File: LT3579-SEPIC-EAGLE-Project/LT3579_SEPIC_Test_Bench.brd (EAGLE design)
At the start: 74 x 58 mm, 160 parts

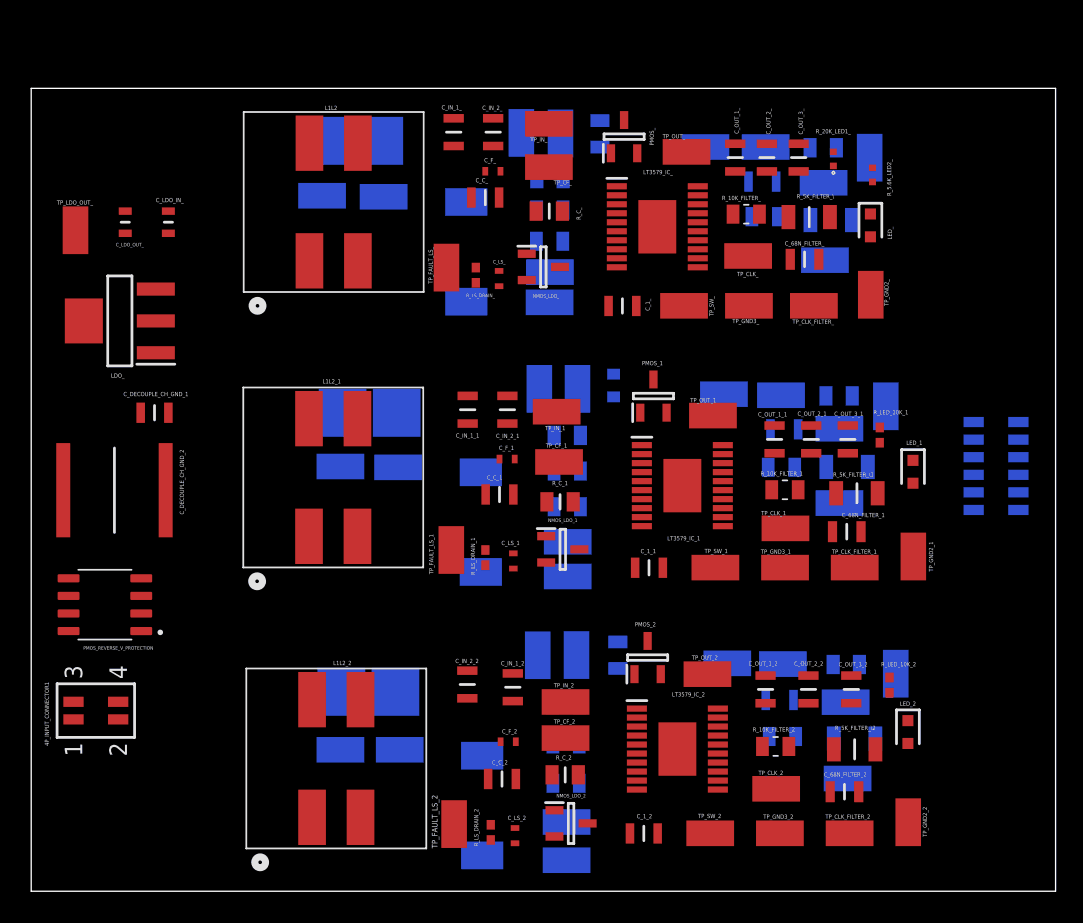
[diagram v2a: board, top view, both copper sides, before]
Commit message: Added new FIles
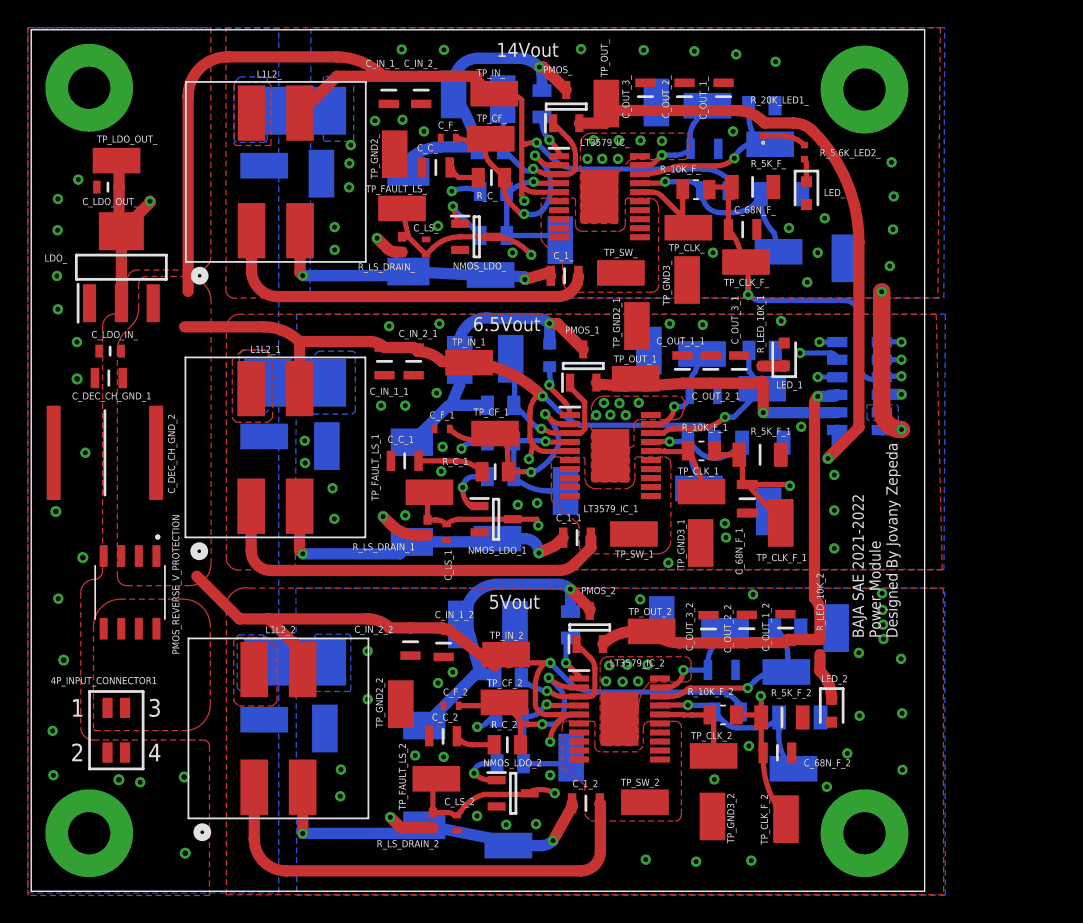
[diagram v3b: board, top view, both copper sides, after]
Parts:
- removed C_68N_FILTER_, C_68N_FILTER_1, C_68N_FILTER_2: CEU4J2X7R1H683K125AE, SamacSys_Parts:CAPC2013X150N
- removed C_DECOUPLE_CH_GND_1: CGA4F4C0G2W222J085AE, SamacSys_Parts:CAPC2012X100N
- removed C_DECOUPLE_CH_GND_2: CGADN3X7R1E476M230LE, SamacSys_Parts:CAPC7563X250N
- removed R_10K_FILTER_, R_10K_FILTER_1, R_10K_FILTER_2: AC0805DR-0710KL, AC0805DR-0710KL:RESC2012X60N
- removed R_5K_FILTER_\, R_5K_FILTER_\1, R_5K_FILTER_\2: RT1206BRD075KL, SamacSys_Parts:RESC3116X65N
- removed TP_CLK_FILTER_, TP_CLK_FILTER_1, TP_CLK_FILTER_2: S1751-46R, S1751-46R:S1751-46R_
- added C_68N_F_, C_68N_F_1, C_68N_F_2: CEU4J2X7R1H683K125AE, SamacSys_Parts:CAPC2013X150N
- added C_DEC_CH_GND_1: CGA4F4C0G2W222J085AE, SamacSys_Parts:CAPC2012X100N
- added C_DEC_CH_GND_2: CGADN3X7R1E476M230LE, SamacSys_Parts:CAPC7563X250N
- added R_10K_F_, R_10K_F_1, R_10K_F_2: AC0805DR-0710KL, AC0805DR-0710KL:RESC2012X60N
- added R_5K_F_, R_5K_F_1, R_5K_F_2: RT1206BRD075KL, SamacSys_Parts:RESC3116X65N
- added TP_CLK_F_, TP_CLK_F_1, TP_CLK_F_2: S1751-46R, S1751-46R:S1751-46R_
- added U$1, U$2, U$3, U$4: THROUGH_HOLE_, THROUGH_HOLE:THROUGH_HOLE
- moved TP_GND2_2 37.6 mm to (26.7, 13.5), turned to 270 degrees
- moved TP_GND2_ 35.9 mm to (26.3, 53.2)
- moved TP_GND2_1 26.0 mm to (43.8, 40.8), turned to 90 degrees
- moved LED_1 12.6 mm to (54.4, 38.8), turned to 90 degrees
- moved C_OUT_3_ 11.9 mm to (44.4, 57.4), turned to 90 degrees
- moved 12P_OUTPUT_CONNECTOR1 11.4 mm to (59.8, 36.5)
- moved TP_GND4_1 11.4 mm to (53.3, 27.4), turned to 90 degrees
- moved C_OUT_3_2 11.2 mm to (48.9, 18.9), turned to 90 degrees
- moved C_LDO_IN_ 10.2 mm to (5.70, 39.0), turned to 180 degrees
- moved TP_SHDN_1 10.2 mm to (48.2, 29.1)
- moved R_LED_10K_1 9.61 mm to (52.8, 37.4), turned to 90 degrees
- moved C_OUT_3_1 9.34 mm to (51.1, 37.7), turned to 90 degrees
- moved C_OUT_2_1 8.84 mm to (49.1, 37.7), turned to 90 degrees
- moved C_OUT_1_1 8.36 mm to (47.0, 37.7), turned to 90 degrees
- moved C_IN_2_1 7.62 mm to (27.6, 38.3)
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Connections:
- removed net 0: C_68N_FILTER_.2, C_68N_FILTER_1.2, C_68N_FILTER_2.2, C_C_.2, C_C_1.2, C_C_2.2, C_F_.2, C_F_1.2, C_F_2.2, C_IN_1_.2, C_IN_1_1.2, C_IN_1_2.2, C_IN_2_.2, C_IN_2_1.2, C_IN_2_2.2, C_LDO_IN_.2, C_LDO_OUT_.2, C_LS_.2, C_LS_1.2, C_LS_2.2, C_OUT_1_.2, C_OUT_1_1.2, C_OUT_1_2.2, C_OUT_2_.2, C_OUT_2_1.2, C_OUT_2_2.2, C_OUT_3_.2, C_OUT_3_1.2, C_OUT_3_2.2, C_SS_.2, C_SS_1.2, C_SS_2.2, L1L2_.4, L1L2_1.4, L1L2_2.4, LED_.2, LED_1.2, LED_2.2, LT3579_IC_.21, LT3579_IC_1.21, LT3579_IC_2.21, NMOS_LDO_.2, NMOS_LDO_1.2, NMOS_LDO_2.2, PMOS_REVERSE_V_PROTECTION.4, R_5K_FILTER_\.2, R_5K_FILTER_\1.2, R_5K_FILTER_\2.2, R_T_.2, R_T_1.2, R_T_2.2, R_UVLO2_.1, R_UVLO2_1.1, R_UVLO2_2.1, TP_GND1_.1, TP_GND1_1.1, TP_GND1_2.1, TP_GND2_.1, TP_GND2_1.1, TP_GND2_2.1, TP_GND3_.1, TP_GND3_1.1, TP_GND3_2.1, TP_GND4_.1, TP_GND4_1.1, TP_GND4_2.1
- removed net GND: 12P_OUTPUT_CONNECTOR1.10, 12P_OUTPUT_CONNECTOR1.12, 12P_OUTPUT_CONNECTOR1.8, LDO_.1, LT3579_IC_.20, LT3579_IC_1.20, LT3579_IC_2.20, R_SHUNT_GND_.2, R_SHUNT_GND_1.2, R_SHUNT_GND_2.2, TP_GND_.1, TP_GND_1.1, TP_GND_2.1
- new net GND_: 12P_OUTPUT_CONNECTOR1.12, C_68N_F_.2, C_C_.2, C_F_.2, C_IN_1_.2, C_IN_2_.2, C_LS_.2, C_OUT_1_.2, C_OUT_2_.2, C_OUT_3_.2, C_SS_.2, L1L2_.4, LED_.2, LT3579_IC_.20, LT3579_IC_.21, NMOS_LDO_.2, R_5K_F_.2, R_SHUNT_GND_.2, R_T_.2, R_UVLO2_.1, TP_GND1_.1, TP_GND2_.1, TP_GND3_.1, TP_GND4_.1, TP_GND_.1
- new net GND_1: 12P_OUTPUT_CONNECTOR1.10, C_68N_F_1.2, C_C_1.2, C_F_1.2, C_IN_1_1.2, C_IN_2_1.2, C_LS_1.2, C_OUT_1_1.2, C_OUT_2_1.2, C_OUT_3_1.2, C_SS_1.2, L1L2_1.4, LED_1.2, LT3579_IC_1.20, LT3579_IC_1.21, NMOS_LDO_1.2, R_5K_F_1.2, R_SHUNT_GND_1.2, R_T_1.2, R_UVLO2_1.1, TP_GND1_1.1, TP_GND2_1.1, TP_GND3_1.1, TP_GND4_1.1, TP_GND_1.1
- new net GND_2: 12P_OUTPUT_CONNECTOR1.8, C_68N_F_2.2, C_C_2.2, C_F_2.2, C_IN_1_2.2, C_IN_2_2.2, C_LS_2.2, C_OUT_1_2.2, C_OUT_2_2.2, C_OUT_3_2.2, C_SS_2.2, L1L2_2.4, LED_2.2, LT3579_IC_2.20, LT3579_IC_2.21, NMOS_LDO_2.2, R_5K_F_2.2, R_SHUNT_GND_2.2, R_T_2.2, R_UVLO2_2.1, TP_GND1_2.1, TP_GND2_2.1, TP_GND3_2.1, TP_GND4_2.1, TP_GND_2.1
- net CH_GND: now also C_DEC_CH_GND_1.1, C_DEC_CH_GND_2.1, C_LDO_IN_.2, C_LDO_OUT_.2, LDO_.1, PMOS_REVERSE_V_PROTECTION.4; no longer C_DECOUPLE_CH_GND_1.1, C_DECOUPLE_CH_GND_2.1
- net CLK_: now also R_10K_F_.1; no longer R_10K_FILTER_.1
- net CLK_1: now also R_10K_F_1.1; no longer R_10K_FILTER_1.1
- net CLK_2: now also R_10K_F_2.1; no longer R_10K_FILTER_2.1
- net CLK_FILTER_OUT_: now also C_68N_F_.1, R_10K_F_.2, R_5K_F_.1, TP_CLK_F_.1; no longer C_68N_FILTER_.1, R_10K_FILTER_.2, R_5K_FILTER_\.1, TP_CLK_FILTER_.1
- net CLK_FILTER_OUT_1: now also C_68N_F_1.1, R_10K_F_1.2, R_5K_F_1.1, TP_CLK_F_1.1; no longer C_68N_FILTER_1.1, R_10K_FILTER_1.2, R_5K_FILTER_\1.1, TP_CLK_FILTER_1.1
- net CLK_FILTER_OUT_2: now also C_68N_F_2.1, R_10K_F_2.2, R_5K_F_2.1, TP_CLK_F_2.1; no longer C_68N_FILTER_2.1, R_10K_FILTER_2.2, R_5K_FILTER_\2.1, TP_CLK_FILTER_2.1
- net VIN: now also C_DEC_CH_GND_1.2, C_DEC_CH_GND_2.2; no longer C_DECOUPLE_CH_GND_1.2, C_DECOUPLE_CH_GND_2.2
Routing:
- net VIN: track 0.00 -> 208.1 mm, vias 0 -> 9
- net LDO_OUT_: track 0.00 -> 91.9 mm, vias 0 -> 4
- net FAULT_LS_OUT_2: track 0.00 -> 52.5 mm, vias 0 -> 2
- net VOUT_: track 0.00 -> 46.3 mm, vias 0 -> 1
- net CLK_FILTER_OUT_2: track 0.00 -> 42.5 mm, vias 0 -> 2
- net FAULT_LS_OUT_: track 0.00 -> 38.0 mm, vias 0 -> 2
- net FAULT_LS_OUT_1: track 0.00 -> 37.0 mm, vias 0 -> 2
- net VOUT_2: track 0.00 -> 35.2 mm, vias 0 -> 1
- net SW1-2_2: track 0.00 -> 33.8 mm
- net SW1-2_1: track 0.00 -> 29.7 mm
- net SW1-2_: track 0.00 -> 27.9 mm
- net CLK_FILTER_OUT_: track 0.00 -> 26.8 mm, vias 0 -> 2
- net CLK_FILTER_OUT_1: track 0.00 -> 25.2 mm, vias 0 -> 2
- net N$5: track 0.00 -> 25.0 mm, vias 0 -> 2
- net N$7: track 0.00 -> 24.3 mm, vias 0 -> 1
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- added copper zone on layer 1, net CH_GND
- added copper zone on layer 16, net CH_GND
- added copper zone on layer 1, net GND_
- added copper zone on layer 16, net GND_
- added copper zone on layer 1, net GND_1
- added copper zone on layer 16, net GND_1
- added copper zone on layer 1, net GND_2
- added copper zone on layer 16, net GND_2
- added copper zone on layer 1, net SW1-2_
- added copper zone on layer 1, net SW1-2_1
- added copper zone on layer 1, net SW1-2_2
- added copper zone on layer 1, net VIN
- added copper zone on layer 1, net VIN_CONNECTOR
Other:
- board size 74 x 58 mm -> 64.5 x 62.2 mm
- board text added: "14Vout"
- board text added: "5Vout"
- board text added: "6.5Vout"
- board text added: "BAJA SAE 2021-2022 Power Module Designed By Jovany Zepeda"
